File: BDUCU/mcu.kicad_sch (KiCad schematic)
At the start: 15 parts, among them SW1 SW_Push, U8 ATmega328-A, Y1 16MHz

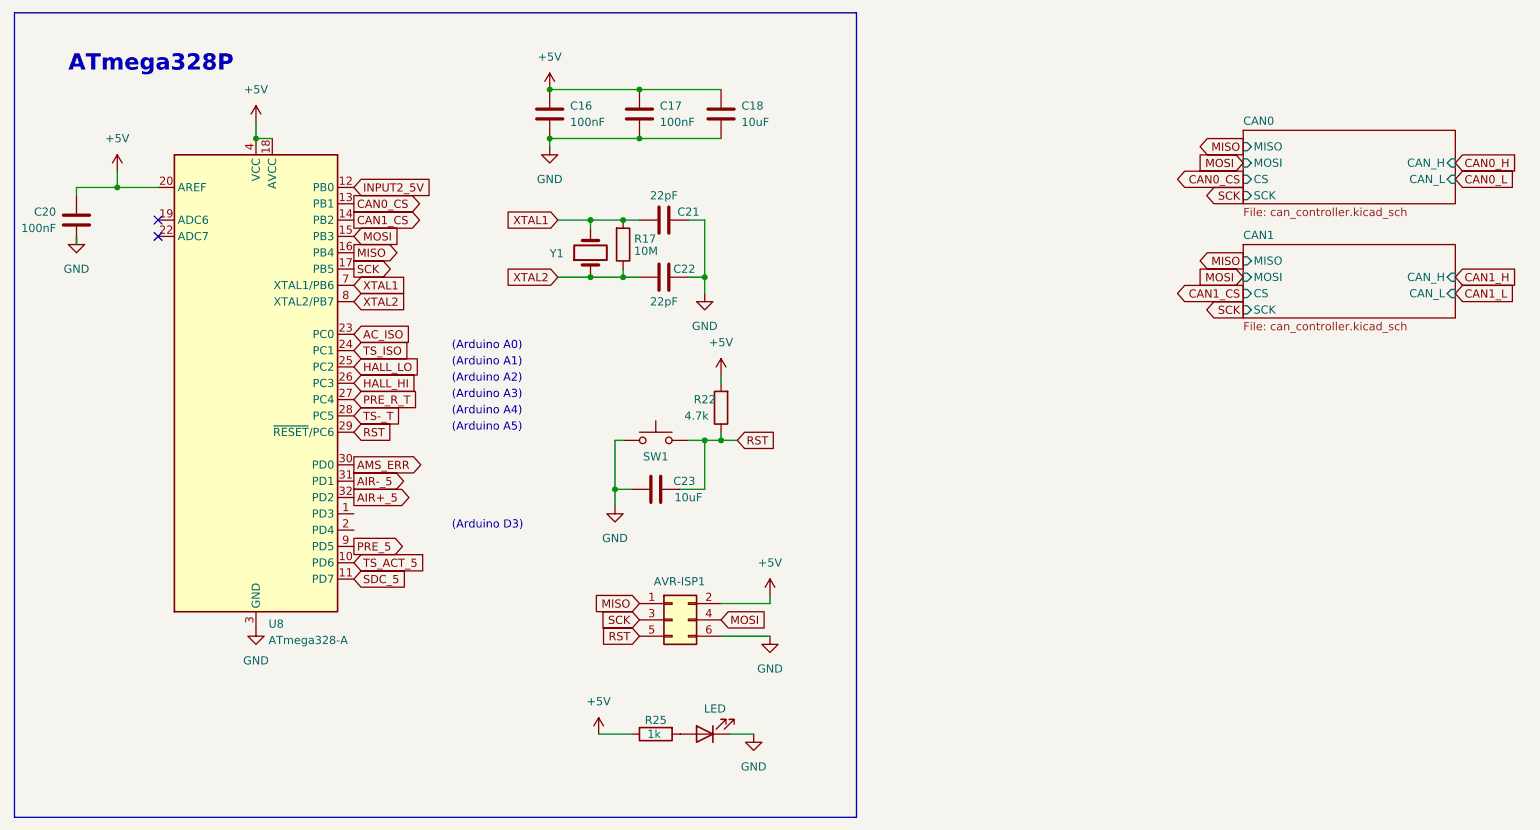
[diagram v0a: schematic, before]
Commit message: I am Nicholas Chan (lesbian version)
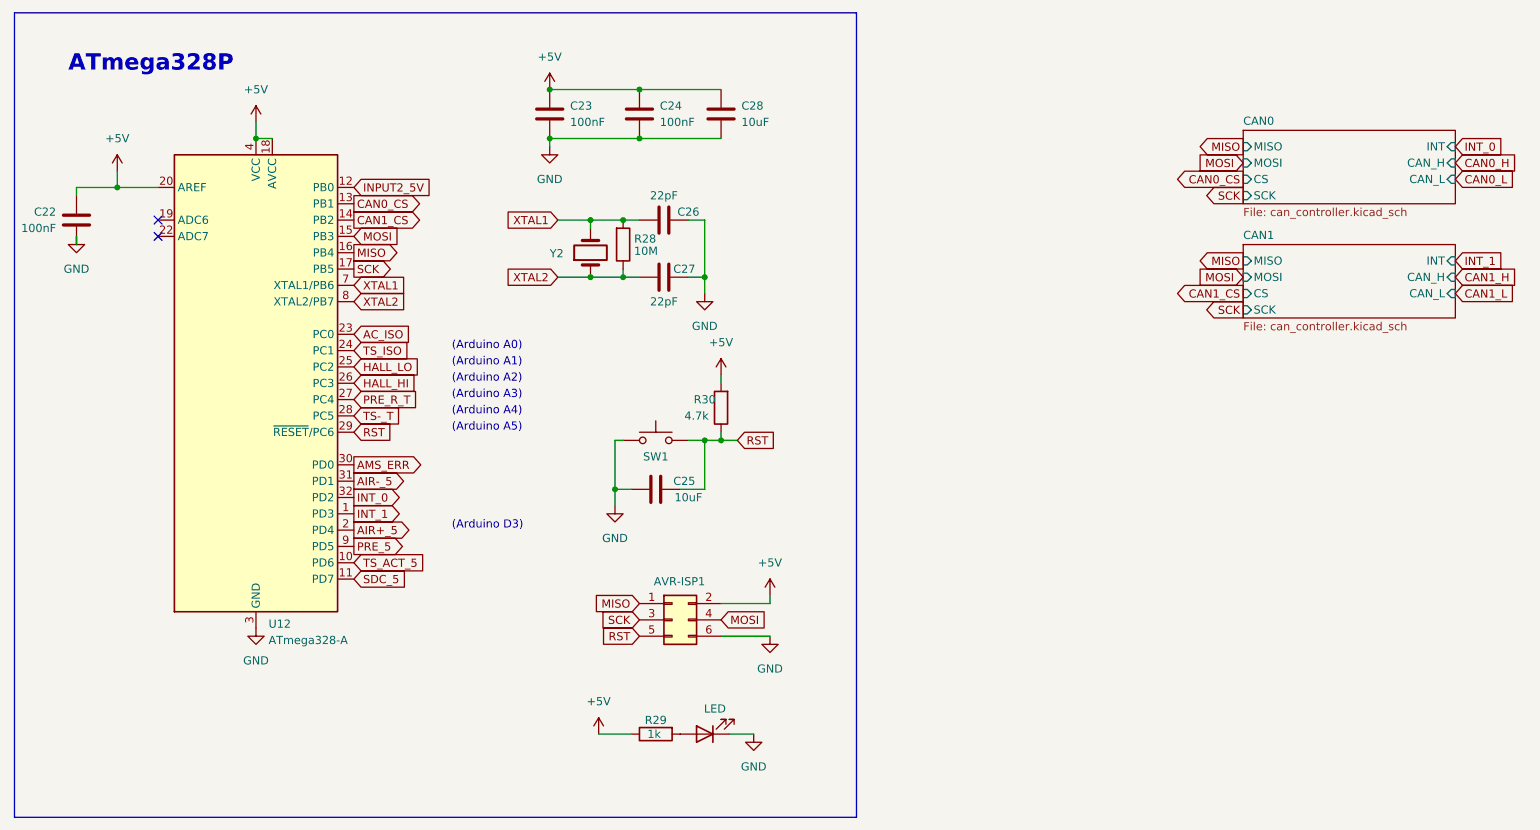
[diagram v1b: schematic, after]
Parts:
- renumbered C20 to C22, C16 to C23, C17 to C24, C23 to C25, C21 to C26, C22 to C27, C18 to C28, R17 to R28, R25 to R29, R22 to R30, U8 to U12, Y1 to Y2
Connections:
- net AIR+_5: now also U12.2 (PD4); no longer U12.32 (PD2)
- net INT_1: now reaches U12.1 (PD3)
- new net INT_0: U12.32 (PD2)
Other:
- sheet CAN0 ports: added INT; removed none
- sheet CAN1 ports: added INT; removed none
